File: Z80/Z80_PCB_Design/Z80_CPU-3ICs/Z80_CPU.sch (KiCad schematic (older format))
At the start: 40 parts, among them J1 USB_B, J2 Conn_01x10, J3 Conn_01x10, U1 Z80CPU, U2 my_components_AS6C4008_PWR, U3 4.9152 MHz, U4 CY8C5267AXI-LP051, U5 MCP23017_SP, Y1 32.768KHz

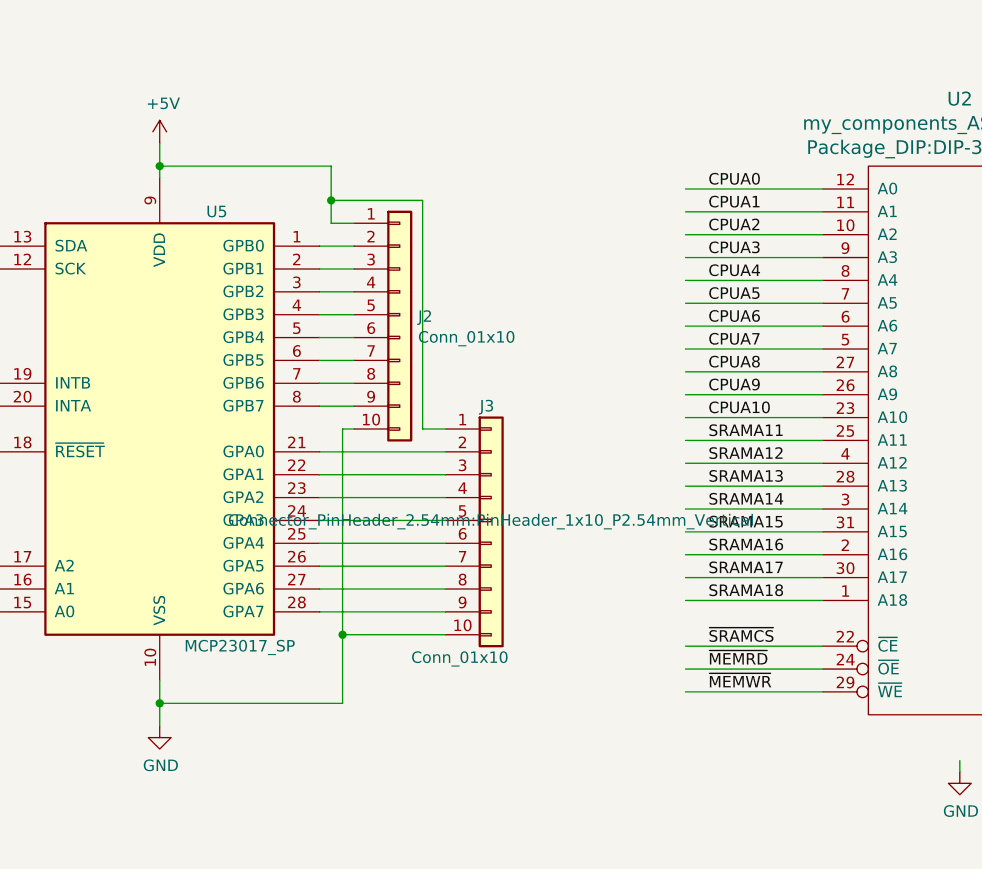
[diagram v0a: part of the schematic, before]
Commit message: z80 cpu legends
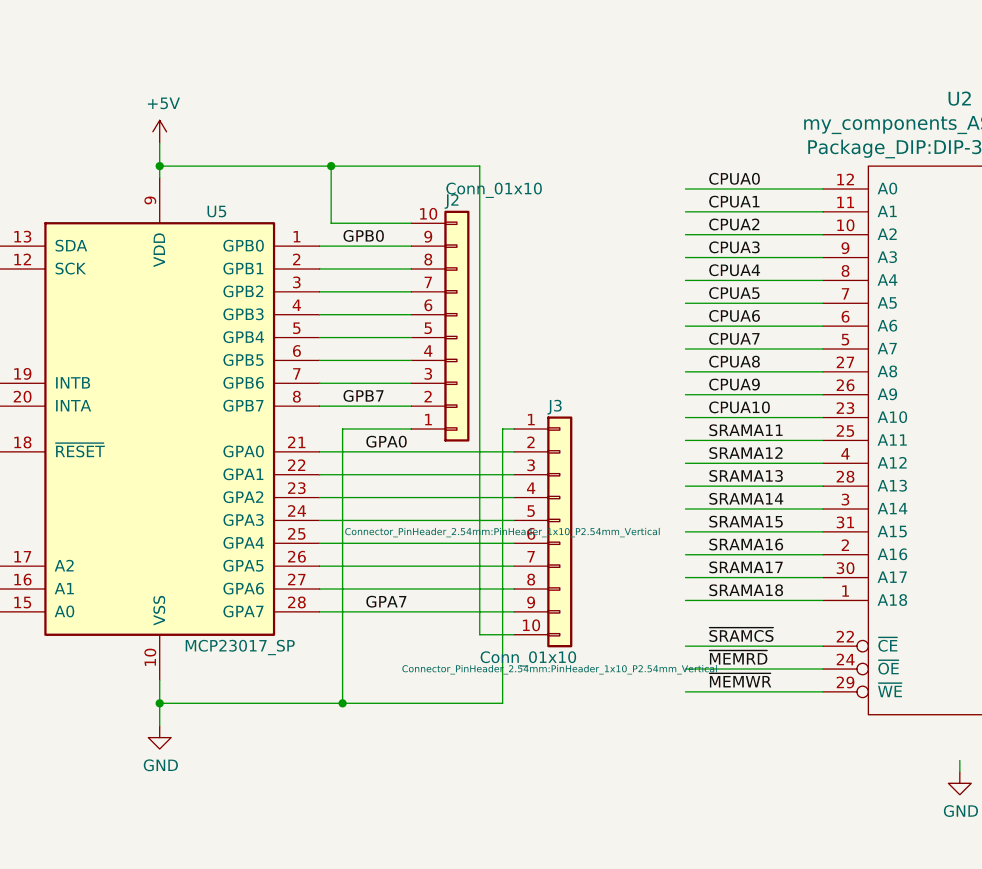
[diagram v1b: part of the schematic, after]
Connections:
- net labels added: GPA0, GPA7, GPB0, GPB7
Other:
- moved on the sheet: J2, J3
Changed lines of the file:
@@
 L Connector_Generic:Conn_01x10 J2
 U 1 1 5D8C51E7
-P 4050 6750
-F 0 "J2" H 4130 6742 50  0000 L CNN
-F 1 "Conn_01x10" H 4130 6651 50  0000 L CNN
-F 2 "Connector_PinHeader_2.54mm:PinHeader_1x10_P2.54mm_Vertical" H 4050 6750 50  0001 C CNN
-F 3 "~" H 4050 6750 50  0001 C CNN
-	1    4050 6750
-	1    0    0    -1
+P 4300 6850
+F 0 "J2" H 4250 6250 50  0000 L CNN
+F 1 "Conn_01x10" H 4250 6200 50  0000 L CNN
+F 2 "Connector_PinHeader_2.54mm:PinHeader_1x10_P2.54mm_Vertical" H 4500 7700 30  0000 C CNN
+F 3 "~" H 4300 6850 50  0001 C CNN
+	1    4300 6850
+	1    0    0    1
 $EndComp
 $Comp
 L Connector_Generic:Conn_01x10 J3
 U 1 1 5D8DE613
-P 4450 7650
-F 0 "J3" H 4400 8150 50  0000 L CNN
-F 1 "Conn_01x10" H 4100 7050 50  0000 L CNN
-F 2 "Connector_PinHeader_2.54mm:PinHeader_1x10_P2.54mm_Vertical" H 4450 7650 50  0000 C CNN
-F 3 "~" H 4450 7650 50  0001 C CNN
-	1    4450 7650
+P 4750 7650
+F 0 "J3" H 4700 8150 50  0000 L CNN
+F 1 "Conn_01x10" H 4400 7050 50  0000 L CNN
+F 2 "Connector_PinHeader_2.54mm:PinHeader_1x10_P2.54mm_Vertical" H 4750 7000 30  0000 C CNN
+F 3 "~" H 4750 7650 50  0001 C CNN
+	1    4750 7650
 	1    0    0    -1
 $EndComp
 Wire Wire Line
-	3700 6450 3850 6450
+	3700 6450 4100 6450
 Wire Wire Line
-	3850 6550 3700 6550
+	4100 6550 3700 6550
 Wire Wire Line
-	3700 6650 3850 6650
+	3700 6650 4100 6650
 Wire Wire Line
-	3700 6750 3850 6750
+	3700 6750 4100 6750
 Wire Wire Line
-	3700 6850 3850 6850
+	3700 6850 4100 6850
 Wire Wire Line
-	3700 6950 3850 6950
+	3700 6950 4100 6950
 Wire Wire Line
-	3700 7050 3850 7050
+	3700 7050 4100 7050
 Wire Wire Line
-	3700 7150 3850 7150
+	3700 7150 4100 7150
 Wire Wire Line
-	3700 7350 4250 7350
+	3700 7350 4550 7350
 Wire Wire Line
-	3700 7450 4250 7450
+	3700 7450 4550 7450
 Wire Wire Line
-	3700 7550 4250 7550
+	3700 7550 4550 7550
 Wire Wire Line
-	3700 7650 4250 7650
+	3700 7650 4550 7650
 Wire Wire Line
-	3700 7750 4250 7750
+	3700 7750 4550 7750
 Wire Wire Line
-	3700 7850 4250 7850
+	3700 7850 4550 7850
 Wire Wire Line
-	3700 7950 4250 7950
+	3700 7950 4550 7950
 Wire Wire Line
-	3700 8050 4250 8050
+	3700 8050 4550 8050
 Wire Wire Line
-	3850 7250 3800 7250
-Wire Wire Line
-	3800 7250 3800 8150
-Wire Wire Line
-	3800 8150 4250 8150
-Wire Wire Line
-	3800 8150 3800 8450
+	4100 7250 3800 7250
 Wire Wire Line
 	3800 8450 3000 8450
 Wire Wire Line
 	3000 8450 3000 8350
-Connection ~ 3800 8150
 Wire Wire Line
 	3000 8450 3000 8550
@@
 $EndComp
 Wire Wire Line
-	4250 7250 4150 7250
+	4400 6100 3750 6100
 Wire Wire Line
-	4150 7250 4150 6250
+	3750 6100 3750 6350
 Wire Wire Line
-	4150 6250 3750 6250
-Wire Wire Line
-	3750 6250 3750 6350
-Wire Wire Line
-	3750 6350 3850 6350
+	3750 6350 4100 6350
 Wire Wire Line
 	3000 6150 3000 6100
 Wire Wire Line
 	3000 6100 3750 6100
-Wire Wire Line
-	3750 6100 3750 6250
-Connection ~ 3750 6250
+Connection ~ 3750 6100
 Wire Wire Line
 	3000 6100 3000 6000
@@
 Text Label 1800 6550 0    50   ~ 0
 SCL
+Text Label 3800 6450 0    50   ~ 0
+GPB0
+Text Label 3800 7150 0    50   ~ 0
+GPB7
+Text Label 3900 7350 0    50   ~ 0
+GPA0
+Text Label 3900 8050 0    50   ~ 0
+GPA7
+Wire Wire Line
+	3800 7250 3800 8450
+Wire Wire Line
+	4550 7250 4500 7250
+Wire Wire Line
+	4500 7250 4500 8450
+Wire Wire Line
+	4500 8450 3800 8450
+Connection ~ 3800 8450
+Wire Wire Line
+	4550 8150 4400 8150
+Wire Wire Line
+	4400 6100 4400 8150
 $EndSCHEMATC
